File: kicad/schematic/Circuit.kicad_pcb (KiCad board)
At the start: 2 copper layers, 70 parts, among them Q1 AO3400A, Q2 AO3400A, Q3 AO3400A, Q4 AO3400A, Q5 AO3400A, Q6 AO3400A, Q7 AO3400A, Q8 AO3400A

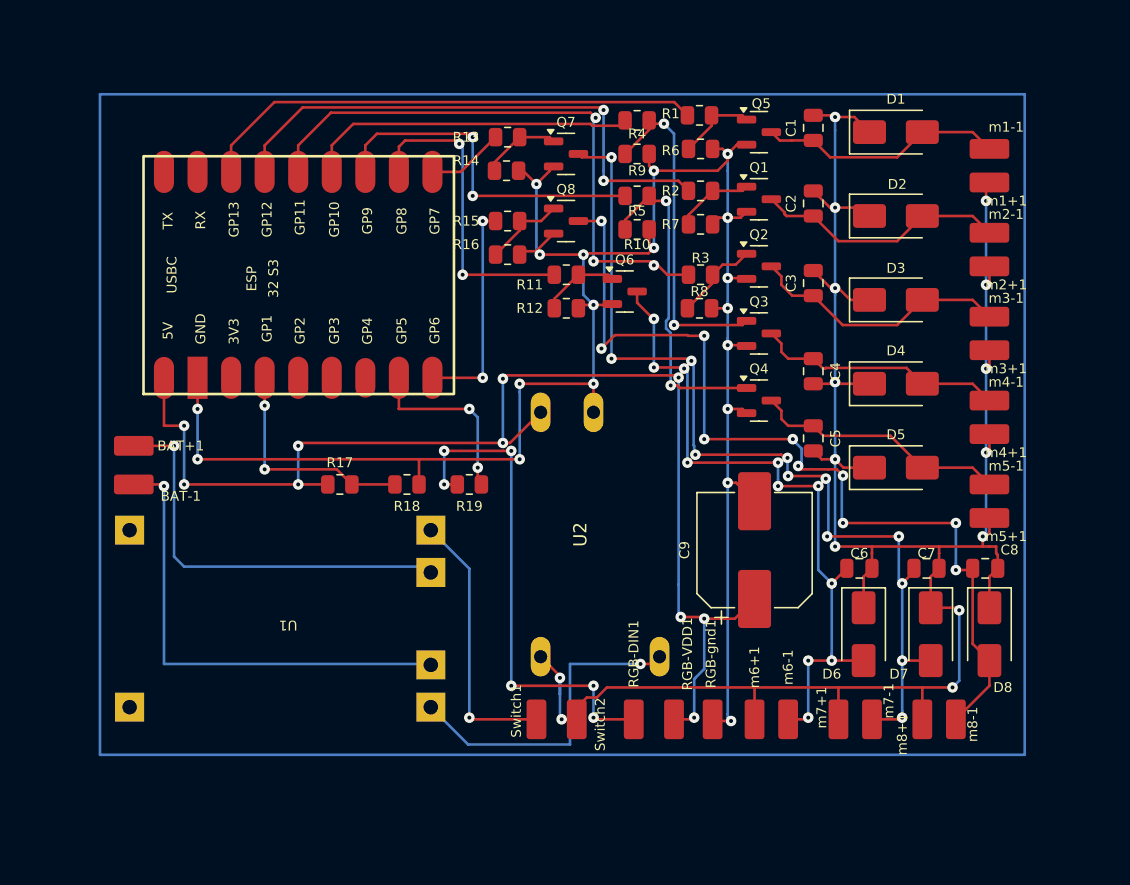
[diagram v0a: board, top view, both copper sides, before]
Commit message: almost final - text image missing
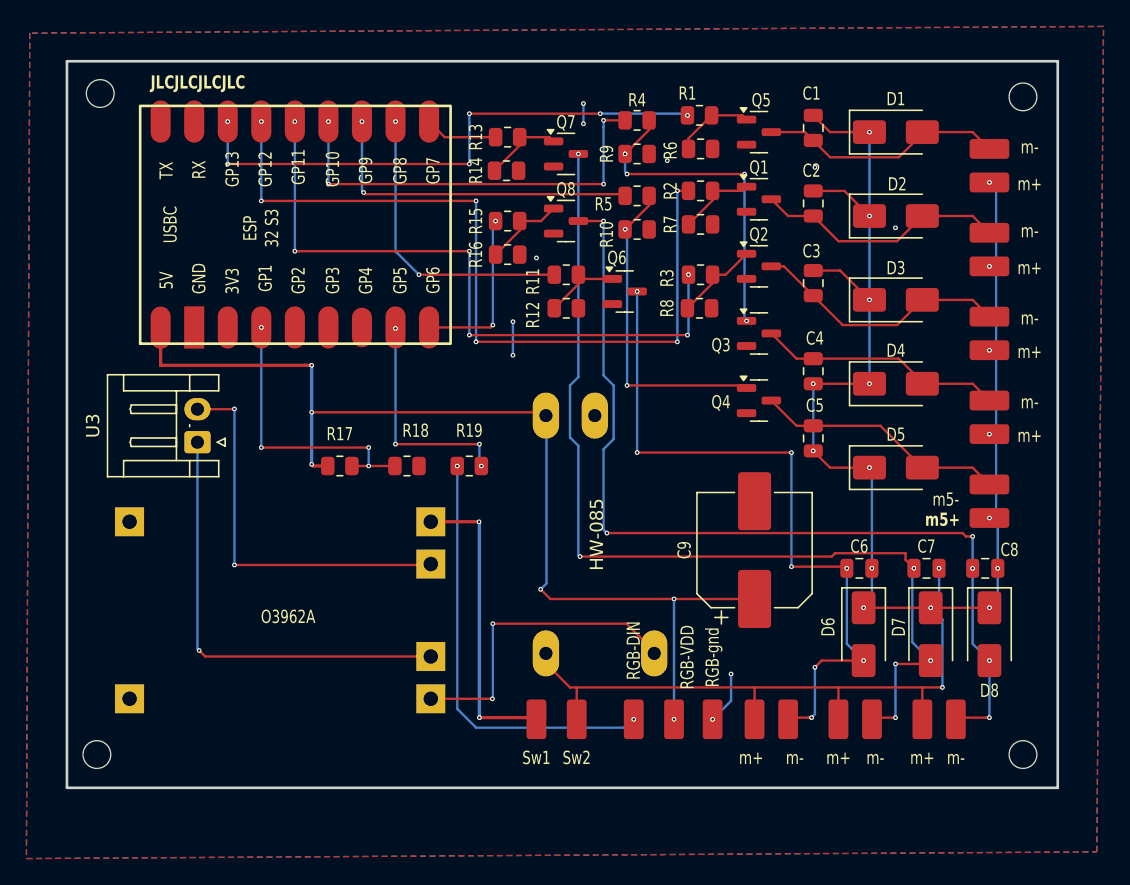
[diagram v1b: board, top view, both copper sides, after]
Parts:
- removed BAT+1, BAT-1: ~, ESP_global:blank pad
- added REF**: MountingHole_2.1mm, MountingHole:MountingHole_2.1mm, F.Cu at (100.8, 87.6)
- added REF**: MountingHole_2.1mm, MountingHole:MountingHole_2.1mm, F.Cu at (30.7, 87.6)
- added REF**: MountingHole_2.1mm, MountingHole:MountingHole_2.1mm, F.Cu at (100.8, 37.8)
- added REF**: MountingHole_2.1mm, MountingHole:MountingHole_2.1mm, F.Cu at (31.0, 37.6)
- added U3: JST-PH2, Connector_JST:JST_EH_S2B-EH_1x02_P2.50mm_Horizontal, F.Cu at (38.3, 64.0)
- moved ESP32_S3_ZERO1 3.82 mm to (45.7, 47.5)
- moved R17 1.40 mm to (49.1, 65.8)
- moved R18 1.40 mm to (54.2, 65.8)
- moved R19 1.40 mm to (58.9, 65.8)
- moved O3962A 0.64 mm to (45.2, 76.7)
- renumbered U2 to HW-085, U1 to O3962A, RGB-DIN1 to RGB-DIN, RGB-VDD1 to RGB-VDD, RGB-gnd1 to RGB-gnd, R1 to RL1, Switch1 to Sw1, Switch2 to Sw2, m7+1 to m+, m8+1 to m+, m3+1 to m+, m6+1 to m+, m4+1 to m+, m2+1 to m+, m1+1 to m+, m1-1 to m-, m7-1 to m-, m3-1 to m-, m2-1 to m-, m4-1 to m-, m8-1 to m-, m6-1 to m-, m5+1 to m5+, m5-1 to m5-
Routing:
- net GND: track 154.1 -> 8.07 mm, vias 19 -> 10
- net Net-(ESP32_S3_ZERO1-GP12): track 41.0 -> 60.4 mm, vias 2 -> 6
- net Net-(D1-K): track 170.9 -> 155.6 mm, vias 15 -> 19
- net Net-(ESP32_S3_ZERO1-5V): track 94.9 -> 80.0 mm, vias 10 -> 6
- net Net-(ESP32_S3_ZERO1-GP10): track 25.1 -> 32.0 mm, vias 0 -> 4
- net Net-(ESP32_S3_ZERO1-GP11): track 44.2 -> 50.5 mm, vias 3 -> 6
- net Net-(RGB-DIN1-pin): track 38.1 -> 32.6 mm, vias 6 -> 2
- net Net-(ESP32_S3_ZERO1-GP1): track 17.3 -> 21.9 mm, vias 2 -> 4
- net Net-(ESP32_S3_ZERO1-GP6): track 16.6 -> 12.9 mm
- net Net-(ESP32_S3_ZERO1-GP13): track 38.3 -> 41.9 mm, vias 0 -> 6
- net Net-(ESP32_S3_ZERO1-GP5): track 13.8 -> 16.9 mm, vias 2 -> 4
- net Net-(Switch1-pin): track 20.5 -> 22.9 mm, vias 1 -> 2
- net Net-(BT1--): track 36.0 -> 34.0 mm
- net Net-(BT1-+): track 31.4 -> 29.5 mm, vias 1 -> 2
- net Net-(ESP32_S3_ZERO1-GP9): track 26.6 -> 25.3 mm
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- added copper zone on B.Cu, net GND
- added copper zone on F.Cu, net GND
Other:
- board outline added: 75 x 55 mm
- board text added: "JLCJLCJLCJLC"
